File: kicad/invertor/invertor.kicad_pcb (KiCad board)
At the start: 2 copper layers, 25.3 x 14.7 mm, 23 parts, among them J1 Conn, J2 Conn, J3 Conn, J4 Conn, J5 Conn, J6 Conn, Q1 IRF7343PBF, Q2 IRF7343PBF, Q3 IRLML6344, Q4 IRLML6344

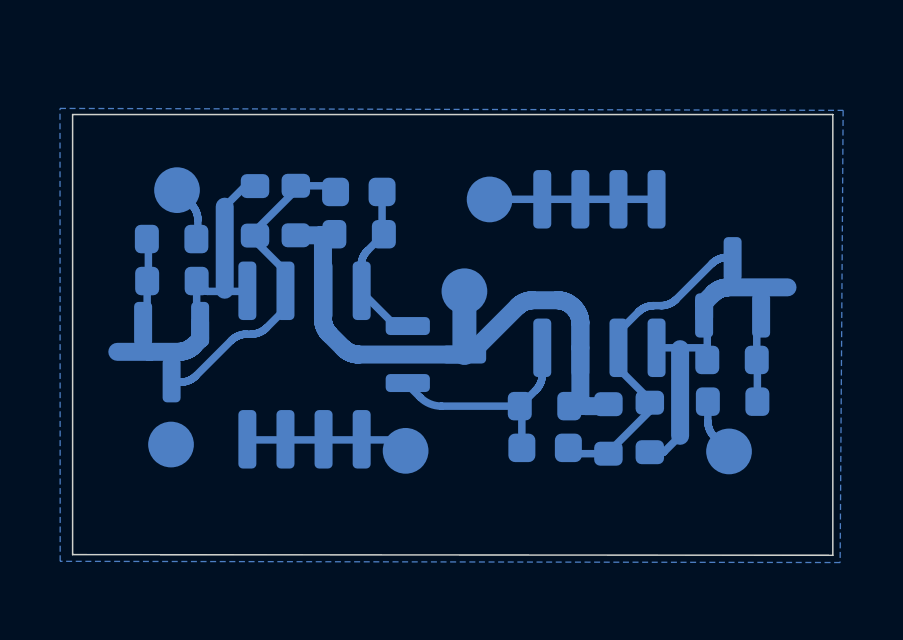
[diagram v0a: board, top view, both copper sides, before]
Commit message: изменено:      kicad/invertor/invertor.kicad_pcb
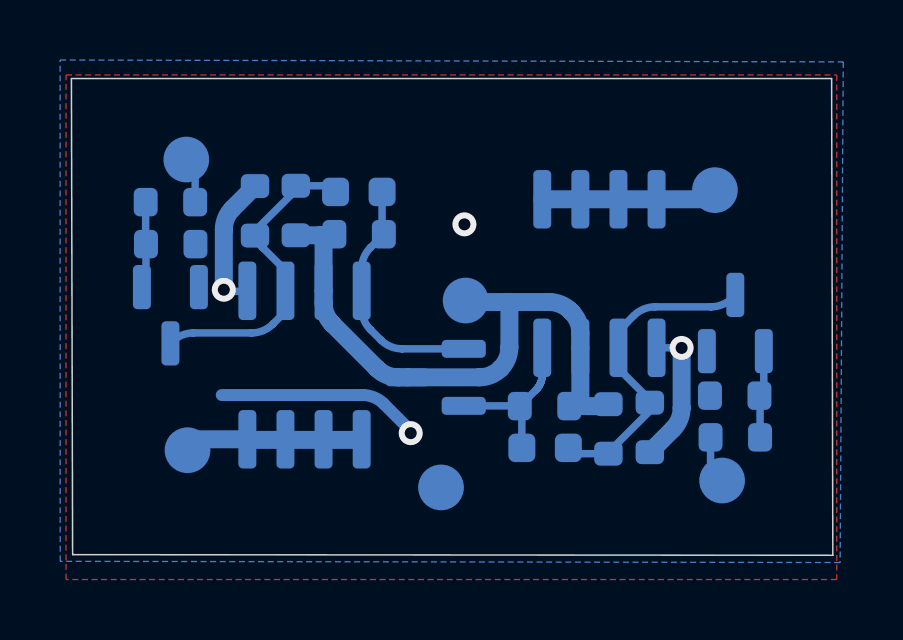
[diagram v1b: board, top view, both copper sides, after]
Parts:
- moved J6 9.11 mm to (42.7, 49.2)
- moved J5 7.52 mm to (51.9, 39.3)
- moved J1 7.27 mm to (34.3, 47.9)
- moved Q3 1.23 mm to (33.7, 43.4)
- moved R8 1.23 mm to (33.7, 41.1)
- moved R6 1.23 mm to (33.7, 39.7)
- moved Q4 1.19 mm to (52.5, 43.7)
- moved R5 1.19 mm to (52.5, 46.1)
- moved R9 1.19 mm to (52.5, 47.5)
- moved J3 1.07 mm to (34.2, 38.2)
- moved J2 1.00 mm to (52.1, 49.0)
- moved D2 0.76 mm to (42.6, 45.5), turned to 180 degrees
- moved J4 0.31 mm to (43.6, 43.0)
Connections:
- D2 pad 1: Net-(C3-Pad1) -> Net-(C1-Pad1)
- D2 pad 2: Net-(C1-Pad1) -> Net-(C3-Pad1)
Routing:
- net GND: track 21.6 -> 16.4 mm, vias 0 -> 4
- net Net-(C1-Pad1): track 5.60 -> 8.27 mm
- net Net-(C3-Pad1): track 7.71 -> 5.52 mm
- net /+12v: track 20.4 -> 21.0 mm
- added copper zone on F.Cu, net GND
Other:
- board size 25.3 x 14.7 mm -> 25.4 x 15.9 mm
